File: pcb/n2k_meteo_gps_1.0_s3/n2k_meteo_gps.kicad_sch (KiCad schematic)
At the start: 30 parts, among them J10 3.3-5V, U2 ESP32-S3_SUPERMINI, U3 MCP2562-E-P, U4 PC817, U5 TSR_1-2450, U6 PC817

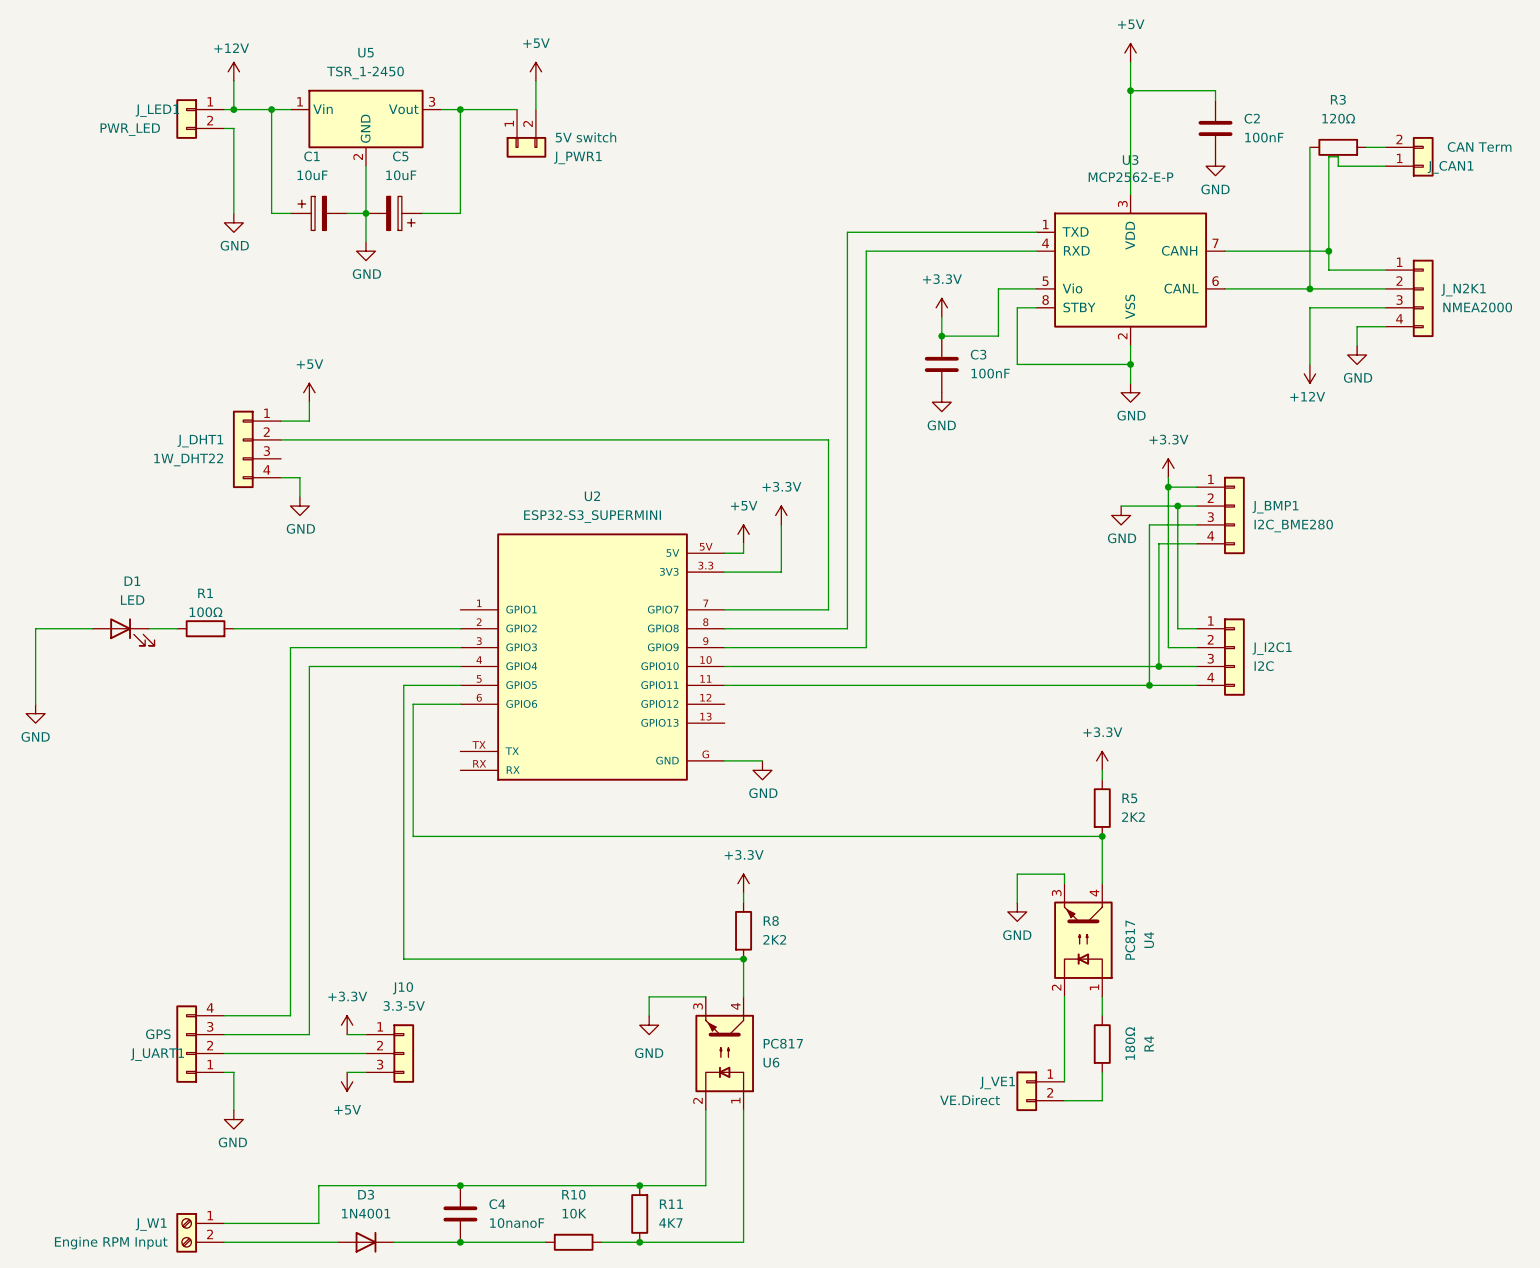
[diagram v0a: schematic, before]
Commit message: PCB
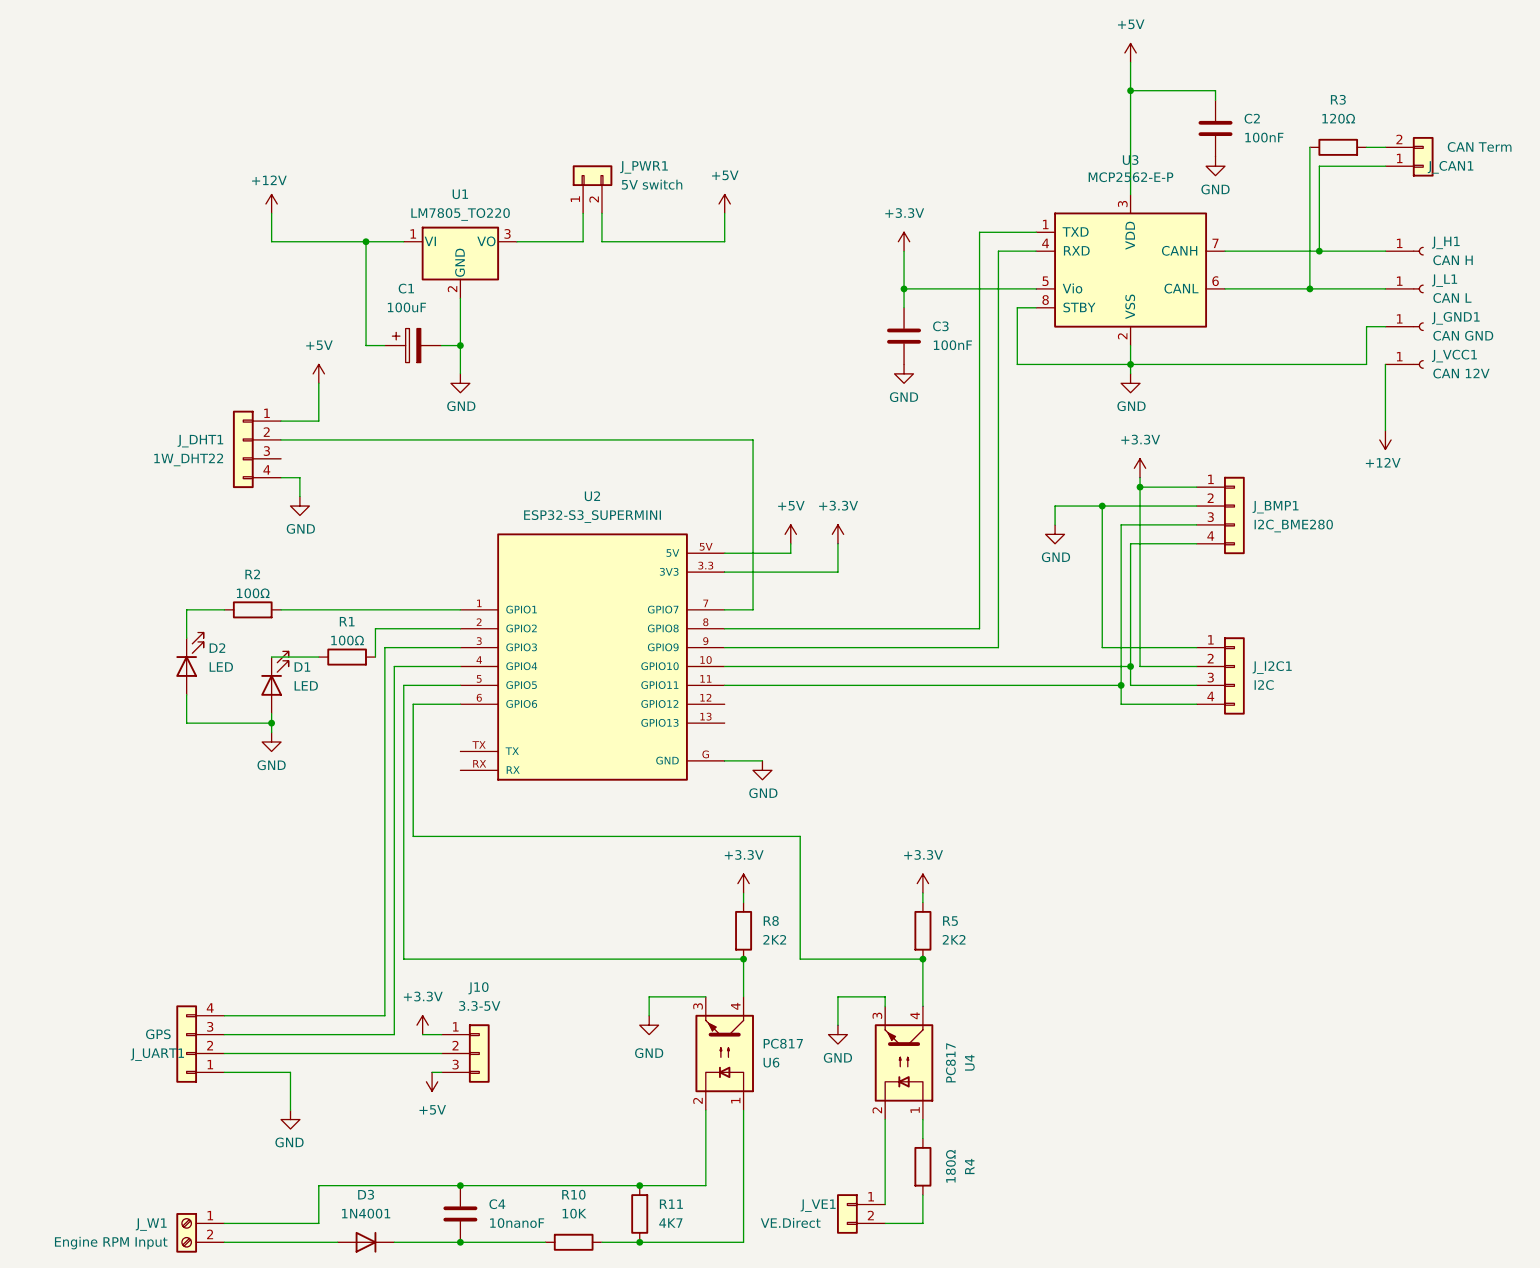
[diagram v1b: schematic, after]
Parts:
- removed C5: 10uF, Capacitor_THT:C_Disc_D4.3mm_W1.9mm_P5.00mm, symbol Device:C_Polarized
- removed J_LED1: PWR_LED, Connector_JST:JST_PH_B2B-PH-K_1x02_P2.00mm_Vertical, symbol Connector_Generic:Conn_01x02
- removed J_N2K1: NMEA2000, Connector_JST:JST_PH_B4B-PH-K_1x04_P2.00mm_Vertical, symbol Connector_Generic:Conn_01x04
- removed U5: TSR_1-2450, Converter_DCDC:Converter_DCDC_TRACO_TSR-1_THT, symbol Regulator_Switching:TSR_1-2450
- added D2: LED, LED_THT:LED_D3.0mm, symbol Device:LED
- added J_GND1: CAN GND, MountingHole:MountingHole_2.2mm_M2_DIN965_Pad_TopBottom, symbol Connector:Conn_01x01_Socket
- added J_H1: CAN H, MountingHole:MountingHole_2.2mm_M2_DIN965_Pad_TopBottom, symbol Connector:Conn_01x01_Socket
- added J_L1: CAN L, MountingHole:MountingHole_2.2mm_M2_DIN965_Pad_TopBottom, symbol Connector:Conn_01x01_Socket
- added J_VCC1: CAN 12V, MountingHole:MountingHole_2.2mm_M2_DIN965_Pad_TopBottom, symbol Connector:Conn_01x01_Socket
- added R2: 100Ω, Resistor_THT:R_Axial_DIN0207_L6.3mm_D2.5mm_P7.62mm_Horizontal, symbol Device:R
- added U1: LM7805_TO220, Package_TO_SOT_THT:TO-220-3_Vertical, symbol Regulator_Linear:LM7805_TO220
- C1: value 10uF -> 100uF; footprint Capacitor_THT:C_Disc_D4.3mm_W1.9mm_P5.00mm -> Capacitor_THT:CP_Radial_D10.0mm_P5.00mm
- J_W1: footprint TerminalBlock:TerminalBlock_bornier-2_P5.08mm -> TerminalBlock_Phoenix:TerminalBlock_Phoenix_MKDS-1,5-2_1x02_P5.00mm_Horizontal
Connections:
- net +12V: now also J_VCC1.1 (Pin_1), U1.1 (VI)
- net GND: now also D2.2 (A), J_GND1.1 (Pin_1), U1.2 (GND)
- net at R3.1, U3.6 (CANL): now also J_L1.1 (Pin_1)
- net at J_CAN1.1 (Pin_1), U3.7 (CANH): now also J_H1.1 (Pin_1)
- net at U2.1 (GPIO1): now also R2.2
- net at J_PWR1.1 (Pin_1): now also U1.3 (VO)
- new net: D2.1 (K), R2.1
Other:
- moved on the sheet: C1, C3, D1, J10, J_I2C1, J_PWR1, J_VE1, R1, R4, R5, U4
